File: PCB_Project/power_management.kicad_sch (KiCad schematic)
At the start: 3 parts, among them J1 Batt_Connector, U5 TSR_1-2433, U6 TSR_1-24120

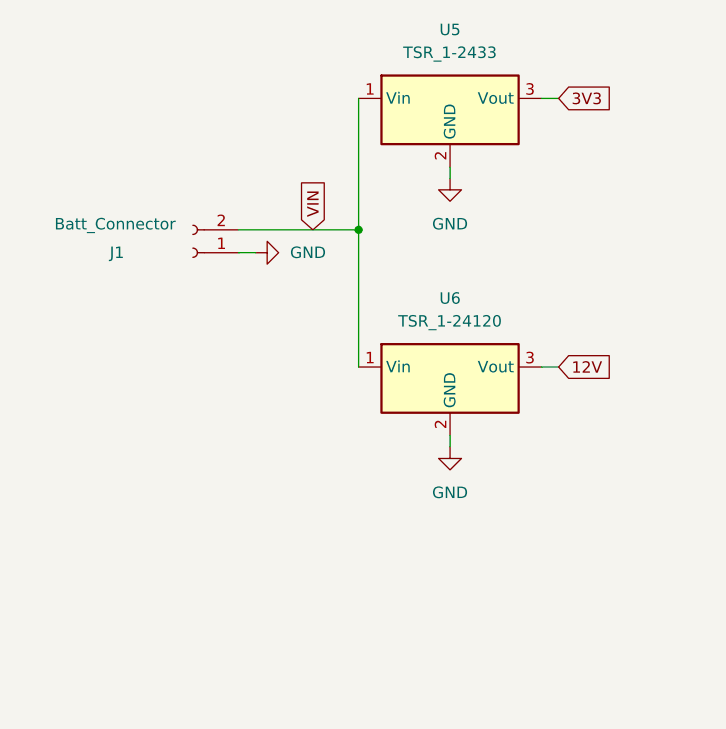
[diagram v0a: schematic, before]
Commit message: done for the day work off this now
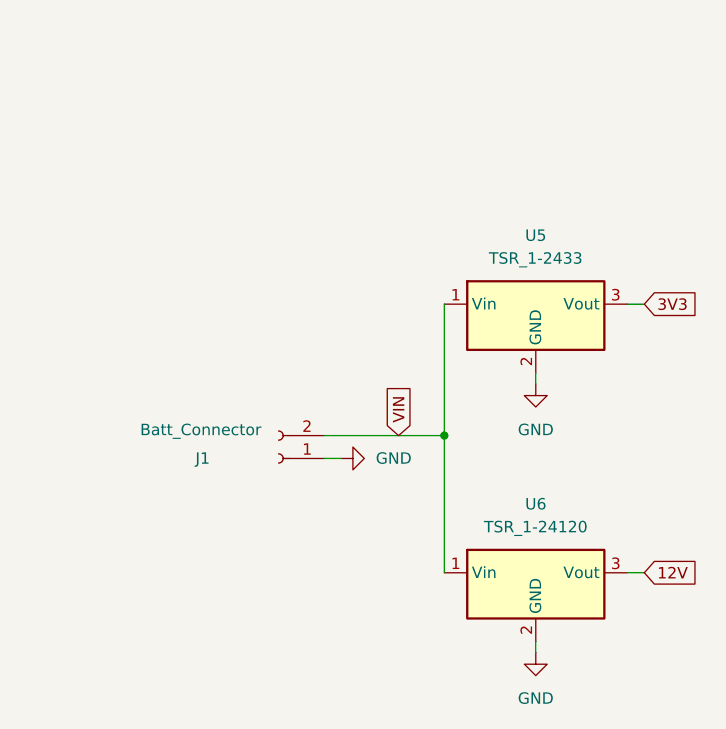
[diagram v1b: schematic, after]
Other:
- moved on the sheet: J1, U5, U6
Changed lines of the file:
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@@
 (kicad_sch (version 20230121) (generator eeschema)
   (paper "A4")
-  (junction (at 109.855 67.945) (diameter 0) (color 0 0 0 0)
+  (junction (at 119.38 90.805) (diameter 0) (color 0 0 0 0)
   )
-  (wire (pts (xy 120.015 60.96) (xy 120.015 62.23))
+  (wire (pts (xy 129.54 83.82) (xy 129.54 85.09))
     (stroke (width 0) (type default))
   )
-  (wire (pts (xy 96.52 70.485) (xy 98.425 70.485))
+  (wire (pts (xy 106.045 93.345) (xy 107.95 93.345))
     (stroke (width 0) (type default))
   )
-  (wire (pts (xy 96.52 67.945) (xy 109.855 67.945))
+  (wire (pts (xy 106.045 90.805) (xy 119.38 90.805))
     (stroke (width 0) (type default))
   )
-  (wire (pts (xy 120.015 90.805) (xy 120.015 92.075))
+  (wire (pts (xy 129.54 113.665) (xy 129.54 114.935))
     (stroke (width 0) (type default))
   )
-  (wire (pts (xy 130.175 53.34) (xy 132.08 53.34))
+  (wire (pts (xy 139.7 76.2) (xy 141.605 76.2))
     (stroke (width 0) (type default))
   )
-  (wire (pts (xy 109.855 67.945) (xy 109.855 83.185))
+  (wire (pts (xy 119.38 90.805) (xy 119.38 106.045))
     (stroke (width 0) (type default))
   )
-  (wire (pts (xy 130.175 83.185) (xy 132.08 83.185))
+  (wire (pts (xy 139.7 106.045) (xy 141.605 106.045))
     (stroke (width 0) (type default))
   )
-  (wire (pts (xy 109.855 67.945) (xy 109.855 53.34))
+  (wire (pts (xy 119.38 90.805) (xy 119.38 76.2))
     (stroke (width 0) (type default))
   )
-  (global_label "3V3" (shape input) (at 132.08 53.34 0) (fields_autoplaced)
+  (global_label "3V3" (shape input) (at 141.605 76.2 0) (fields_autoplaced)
     (effects (font (size 1.27 1.27)) (justify left))
-    (property "Intersheetrefs" "${INTERSHEET_REFS}" (at 138.4934 53.34 0)
+    (property "Intersheetrefs" "${INTERSHEET_REFS}" (at 148.0184 76.2 0)
       (effects (font (size 1.27 1.27)) (justify left) hide)
     )
   )
-  (global_label "VIN" (shape input) (at 104.775 67.945 90) (fields_autoplaced)
+  (global_label "VIN" (shape input) (at 114.3 90.805 90) (fields_autoplaced)
     (effects (font (size 1.27 1.27)) (justify left))
-    (property "Intersheetrefs" "${INTERSHEET_REFS}" (at 104.775 62.0153 90)
+    (property "Intersheetrefs" "${INTERSHEET_REFS}" (at 114.3 84.8753 90)
       (effects (font (size 1.27 1.27)) (justify left) hide)
     )
   )
-  (global_label "12V" (shape input) (at 132.08 83.185 0) (fields_autoplaced)
+  (global_label "12V" (shape input) (at 141.605 106.045 0) (fields_autoplaced)
     (effects (font (size 1.27 1.27)) (justify left))
-    (property "Intersheetrefs" "${INTERSHEET_REFS}" (at 138.4934 83.185 0)
+    (property "Intersheetrefs" "${INTERSHEET_REFS}" (at 148.0184 106.045 0)
       (effects (font (size 1.27 1.27)) (justify left) hide)
     )
   )
-  (symbol (lib_id "Regulator_Switching:TSR_1-24120") (at 120.015 85.725 0) (unit 1)
+  (symbol (lib_id "Regulator_Switching:TSR_1-24120") (at 129.54 108.585 0) (unit 1)
     (in_bom yes) (on_board yes) (dnp no)
-    (property "Reference" "U6" (at 120.015 75.565 0)
+    (property "Reference" "U6" (at 129.54 98.425 0)
       (effects (font (size 1.27 1.27)))
     )
-    (property "Value" "TSR_1-24120" (at 120.015 78.105 0)
+    (property "Value" "TSR_1-24120" (at 129.54 100.965 0)
       (effects (font (size 1.27 1.27)))
     )
-    (property "Footprint" "Converter_DCDC:Converter_DCDC_TRACO_TSR-1_THT" (at 120.015 89.535 0)
+    (property "Footprint" "Converter_DCDC:Converter_DCDC_TRACO_TSR-1_THT" (at 129.54 112.395 0)
       (effects (font (size 1.27 1.27) italic) (justify left) hide)
     )
-    (property "Datasheet" "http://www.tracopower.com/products/tsr1.pdf" (at 120.015 85.725 0)
+    (property "Datasheet" "http://www.tracopower.com/products/tsr1.pdf" (at 129.54 108.585 0)
       (effects (font (size 1.27 1.27)) hide)
     )
@@
     )
   )
-  (symbol (lib_id "Regulator_Switching:TSR_1-2433") (at 120.015 55.88 0) (unit 1)
+  (symbol (lib_id "Regulator_Switching:TSR_1-2433") (at 129.54 78.74 0) (unit 1)
     (in_bom yes) (on_board yes) (dnp no) (fields_autoplaced)
-    (property "Reference" "U5" (at 120.015 45.72 0)
+    (property "Reference" "U5" (at 129.54 68.58 0)
       (effects (font (size 1.27 1.27)))
     )
-    (property "Value" "TSR_1-2433" (at 120.015 48.26 0)
+    (property "Value" "TSR_1-2433" (at 129.54 71.12 0)
       (effects (font (size 1.27 1.27)))
     )
-    (property "Footprint" "Converter_DCDC:Converter_DCDC_TRACO_TSR-1_THT" (at 120.015 59.69 0)
+    (property "Footprint" "Converter_DCDC:Converter_DCDC_TRACO_TSR-1_THT" (at 129.54 82.55 0)
       (effects (font (size 1.27 1.27) italic) (justify left) hide)
     )
-    (property "Datasheet" "http://www.tracopower.com/products/tsr1.pdf" (at 120.015 55.88 0)
+    (property "Datasheet" "http://www.tracopower.com/products/tsr1.pdf" (at 129.54 78.74 0)
       (effects (font (size 1.27 1.27)) hide)
     )
@@
     )
   )
-  (symbol (lib_id "power:GND") (at 120.015 62.23 0) (unit 1)
+  (symbol (lib_id "power:GND") (at 129.54 85.09 0) (unit 1)
     (in_bom yes) (on_board yes) (dnp no) (fields_autoplaced)
-    (property "Reference" "#PWR012" (at 120.015 68.58 0)
+    (property "Reference" "#PWR012" (at 129.54 91.44 0)
       (effects (font (size 1.27 1.27)) hide)
     )
-    (property "Value" "GND" (at 120.015 67.31 0)
+    (property "Value" "GND" (at 129.54 90.17 0)
       (effects (font (size 1.27 1.27)))
     )
-    (property "Footprint" "" (at 120.015 62.23 0)
+    (property "Footprint" "" (at 129.54 85.09 0)
       (effects (font (size 1.27 1.27)) hide)
     )
-    (property "Datasheet" "" (at 120.015 62.23 0)
+    (property "Datasheet" "" (at 129.54 85.09 0)
       (effects (font (size 1.27 1.27)) hide)
     )
@@
     )
   )
-  (symbol (lib_id "power:GND") (at 120.015 92.075 0) (unit 1)
+  (symbol (lib_id "power:GND") (at 129.54 114.935 0) (unit 1)
     (in_bom yes) (on_board yes) (dnp no) (fields_autoplaced)
-    (property "Reference" "#PWR013" (at 120.015 98.425 0)
+    (property "Reference" "#PWR013" (at 129.54 121.285 0)
       (effects (font (size 1.27 1.27)) hide)
     )
-    (property "Value" "GND" (at 120.015 97.155 0)
+    (property "Value" "GND" (at 129.54 120.015 0)
       (effects (font (size 1.27 1.27)))
     )
-    (property "Footprint" "" (at 120.015 92.075 0)
+    (property "Footprint" "" (at 129.54 114.935 0)
       (effects (font (size 1.27 1.27)) hide)
     )
-    (property "Datasheet" "" (at 120.015 92.075 0)
+    (property "Datasheet" "" (at 129.54 114.935 0)
       (effects (font (size 1.27 1.27)) hide)
     )
@@
     )
   )
-  (symbol (lib_id "power:GND") (at 98.425 70.485 90) (unit 1)
+  (symbol (lib_id "power:GND") (at 107.95 93.345 90) (unit 1)
     (in_bom yes) (on_board yes) (dnp no)
-    (property "Reference" "#PWR011" (at 104.775 70.485 0)
+    (property "Reference" "#PWR011" (at 114.3 93.345 0)
       (effects (font (size 1.27 1.27)) hide)
     )
-    (property "Value" "GND" (at 102.235 70.485 90)
+    (property "Value" "GND" (at 111.76 93.345 90)
       (effects (font (size 1.27 1.27)) (justify right))
     )
-    (property "Footprint" "" (at 98.425 70.485 0)
+    (property "Footprint" "" (at 107.95 93.345 0)
       (effects (font (size 1.27 1.27)) hide)
     )
-    (property "Datasheet" "" (at 98.425 70.485 0)
+    (property "Datasheet" "" (at 107.95 93.345 0)
       (effects (font (size 1.27 1.27)) hide)
     )
@@
     )
   )
-  (symbol (lib_id "Connector:Conn_01x02_Socket") (at 91.44 70.485 180) (unit 1)
+  (symbol (lib_id "Connector:Conn_01x02_Socket") (at 100.965 93.345 180) (unit 1)
     (in_bom yes) (on_board yes) (dnp no)
-    (property "Reference" "J1" (at 83.82 70.485 0)
+    (property "Reference" "J1" (at 93.345 93.345 0)
       (effects (font (size 1.27 1.27)) (justify left))
     )
-    (property "Value" "Batt_Connector" (at 89.535 67.31 0)
+    (property "Value" "Batt_Connector" (at 99.06 90.17 0)
       (effects (font (size 1.27 1.27)) (justify left))
     )
-    (property "Footprint" "" (at 91.44 70.485 0)
+    (property "Footprint" "" (at 100.965 93.345 0)
       (effects (font (size 1.27 1.27)) hide)
     )
-    (property "Datasheet" "~" (at 91.44 70.485 0)
+    (property "Datasheet" "~" (at 100.965 93.345 0)
       (effects (font (size 1.27 1.27)) hide)
     )
